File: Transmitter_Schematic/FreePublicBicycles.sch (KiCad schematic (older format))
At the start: 43 parts, among them J1 Conn_01x04_Female, Q1 PN2222A, Q2 IRF4905, SW1 Button, U1 ATmega328-PU, U2 MP1584, U3 BA33BC0T, U4 S9V11F5, U5 RFM95W-868S2, U6 NEO-6M, Y1 16MHz

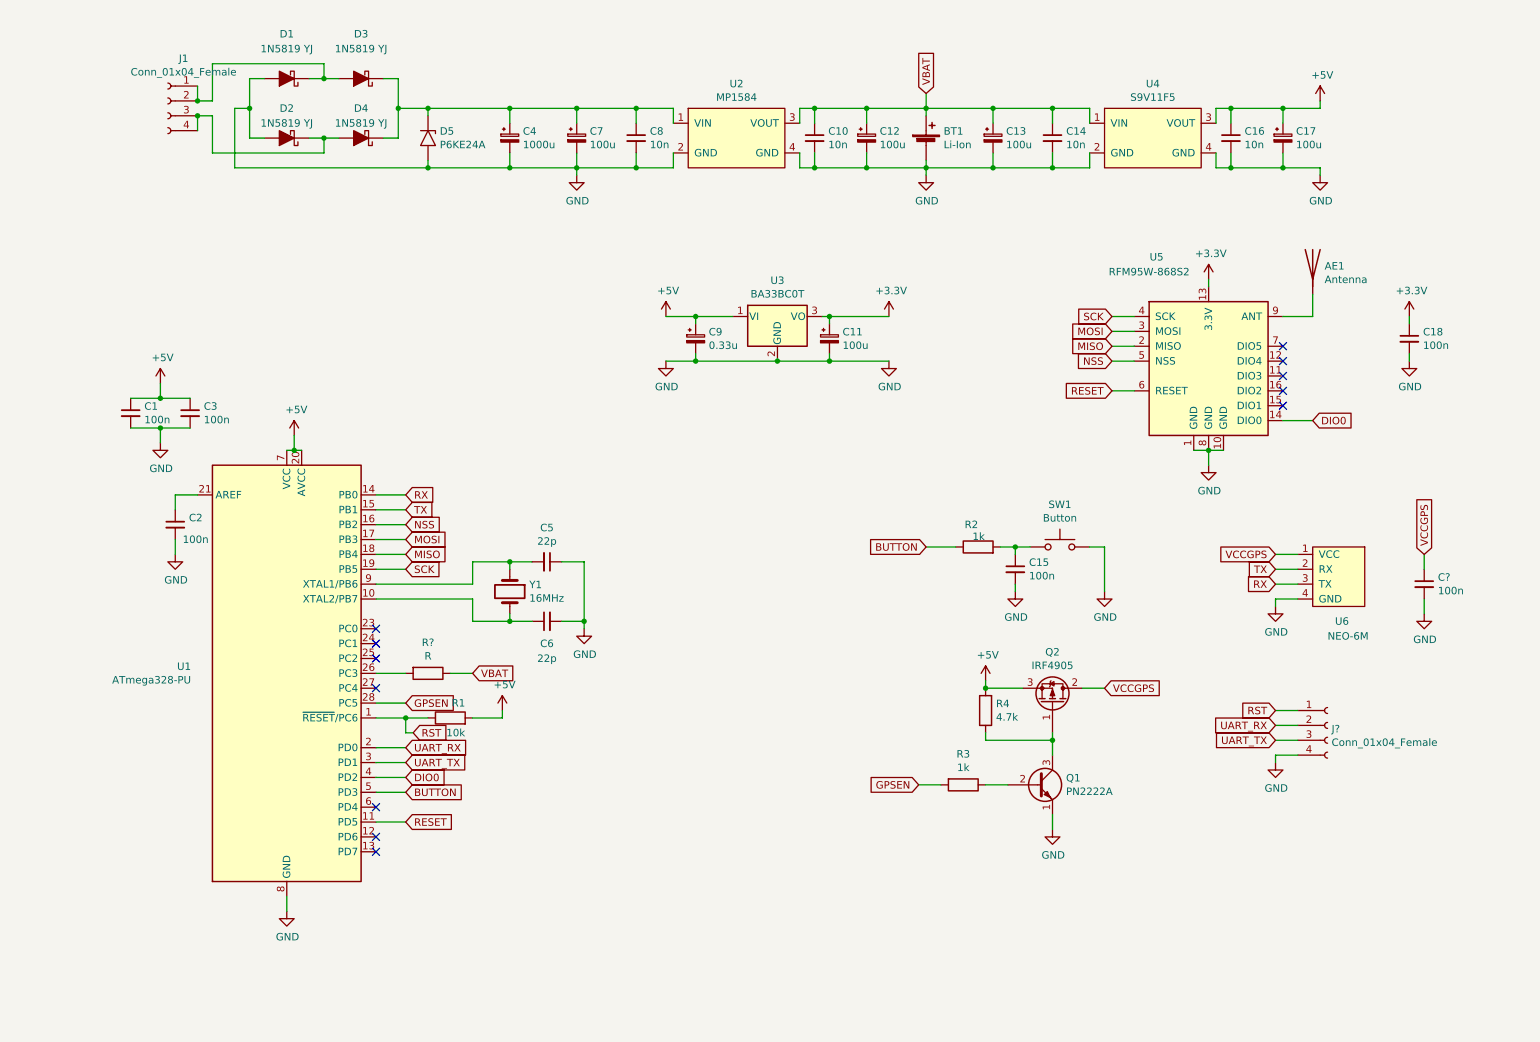
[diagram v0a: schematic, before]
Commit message: Added changes to schematics
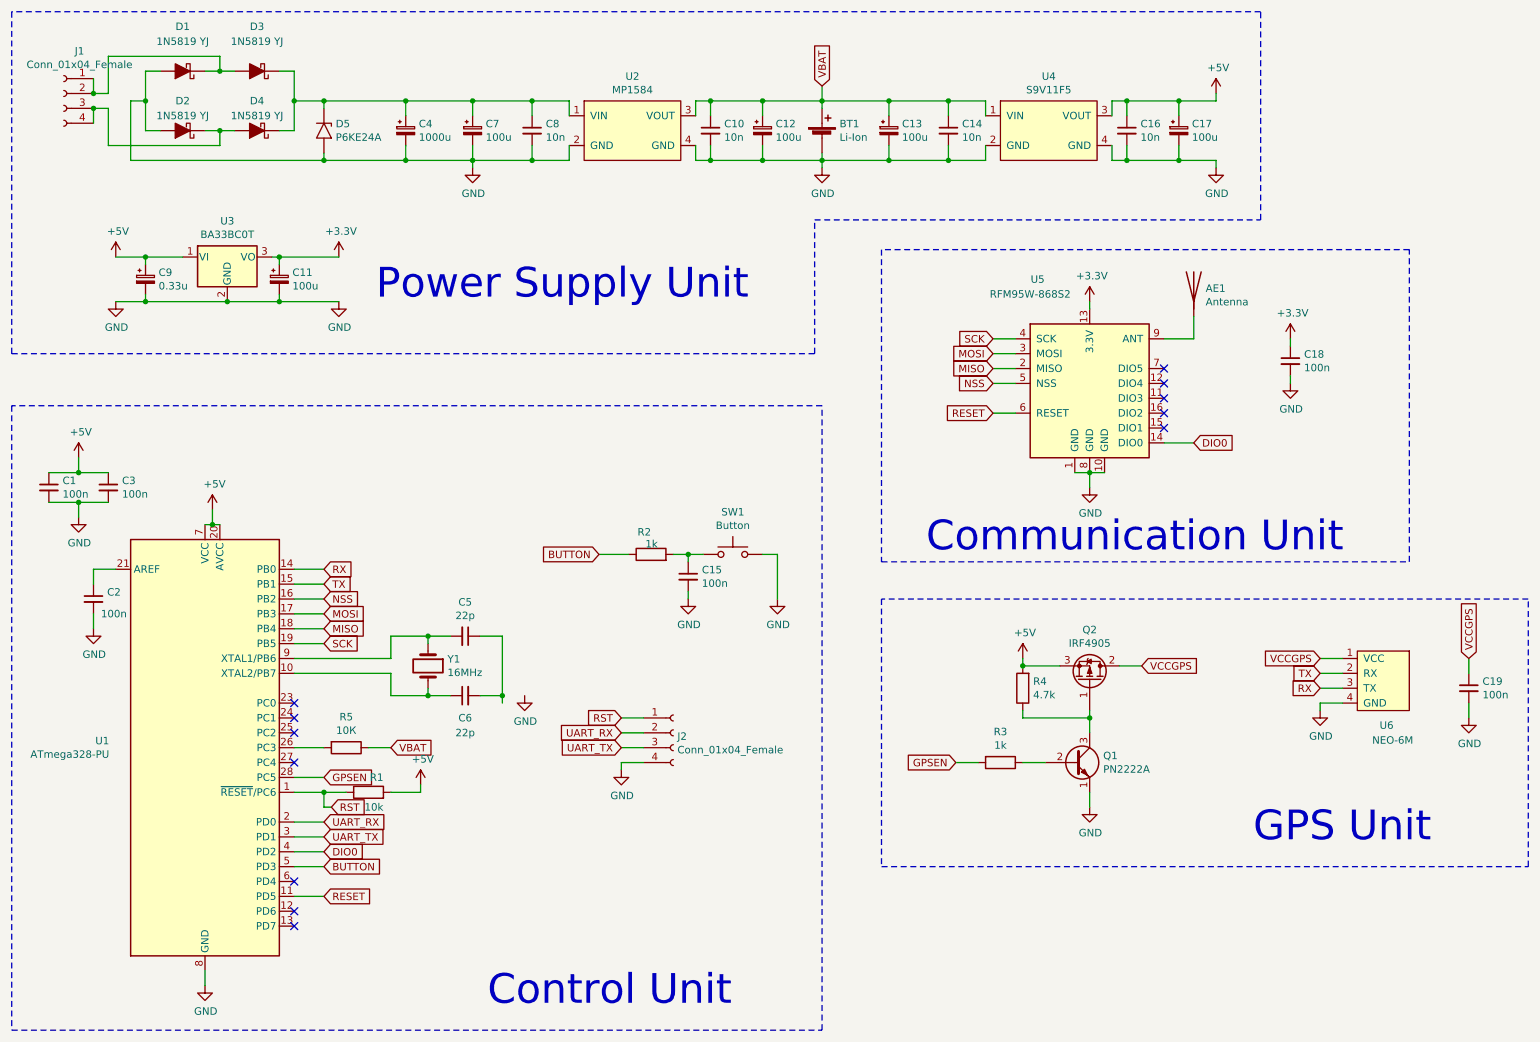
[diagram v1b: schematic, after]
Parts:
- R5: renamed from R?; value R -> 10К
- gave numbers to parts that had none: 2
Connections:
- net GND: no longer C5.1, C6.2
- new net: C5.1, C6.2
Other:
- note added: "Communication Unit"
- note added: "Control Unit"
- note added: "GPS Unit"
- note added: "Power Supply Unit"
- moved on the sheet: AE1, BT1, C1, C10, C11, C12, C13, C14, C15, C16, C17, C18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
